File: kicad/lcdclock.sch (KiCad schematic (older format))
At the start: 26 parts, among them J1 Conn_JLink_SWD, Q1 BSH205, SW1 SW_Push, U1 STM32L073xx_48, U2 ELV_DCF-2, U3 TPS70630, U4 LCD, Y1 32.768kHz 12.5pF

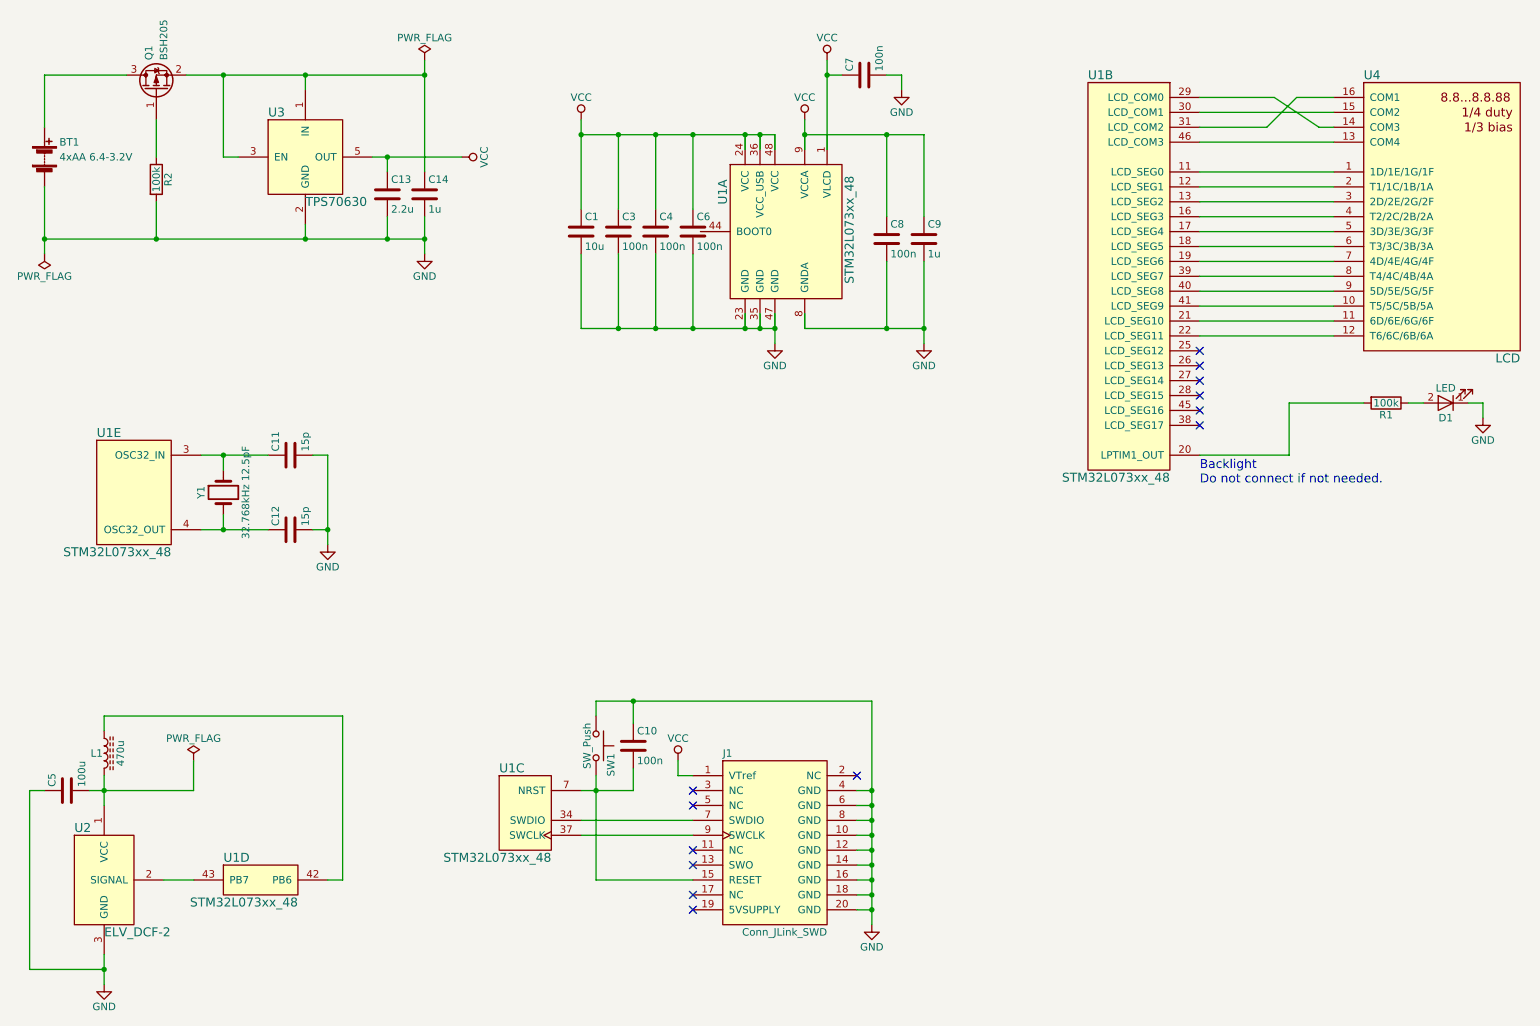
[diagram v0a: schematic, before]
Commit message: Final fixes
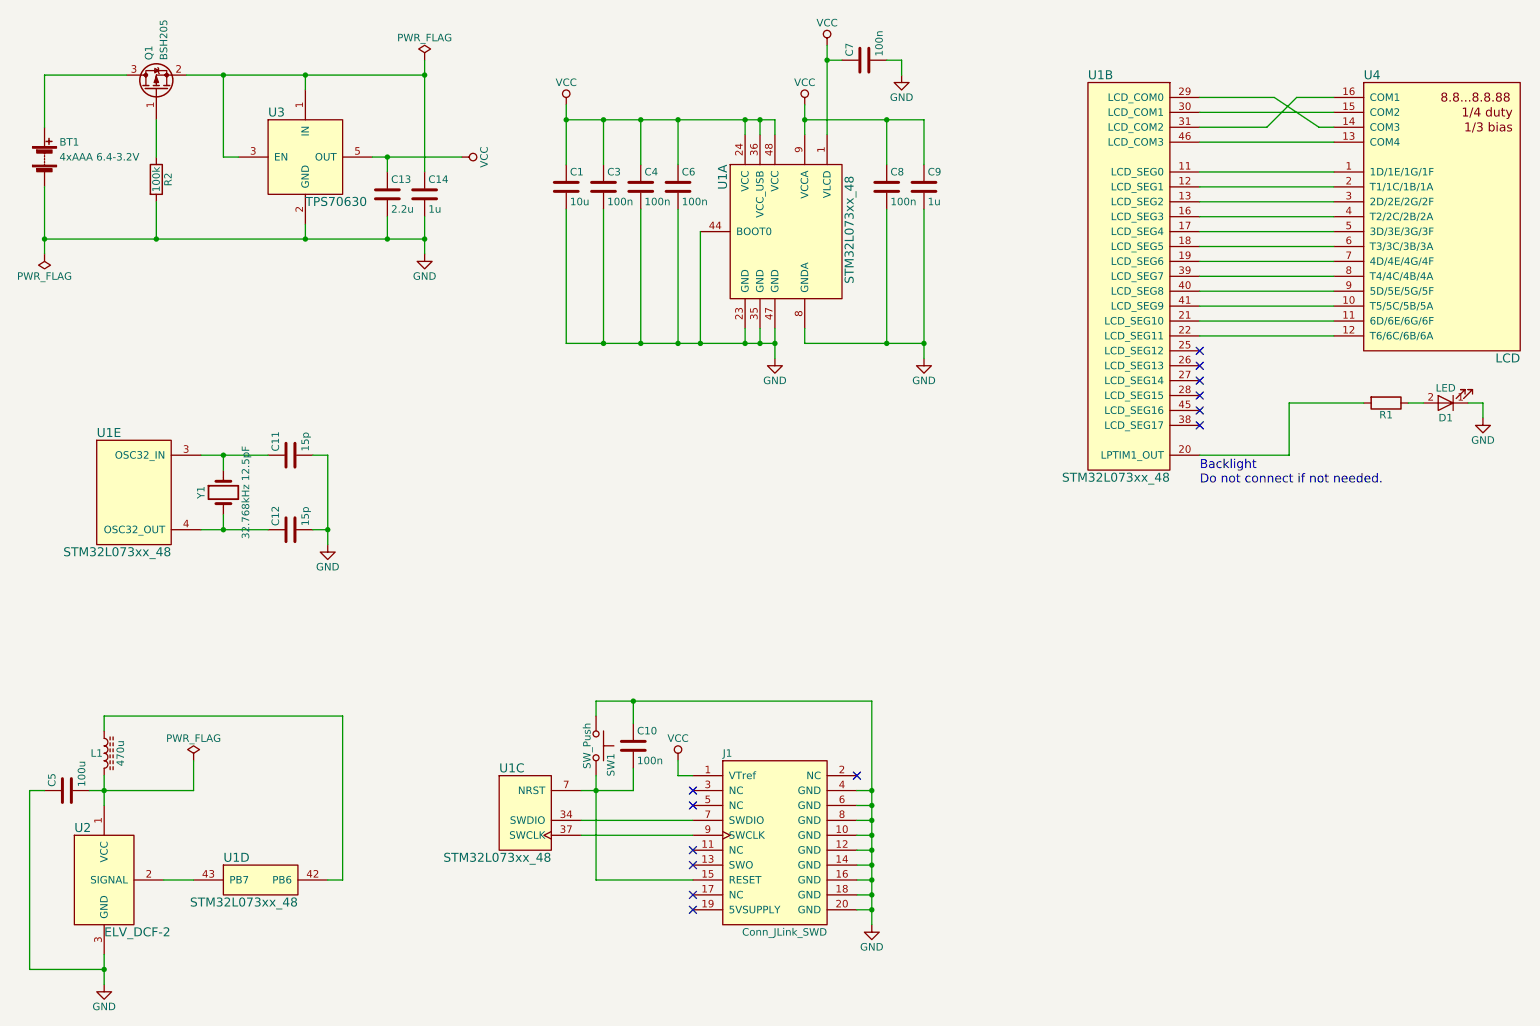
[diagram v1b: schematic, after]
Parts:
- BT1: value 4xAA 6.4-3.2V -> 4xAAA 6.4-3.2V
- R1: value 100k -> ?
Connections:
- wire segments 110 -> 111
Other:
- moved on the sheet: C1, C3, C4, C6, C7, C8, C9
